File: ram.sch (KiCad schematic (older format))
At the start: 7 parts, among them U1 LFE5U-85F-6BG381C

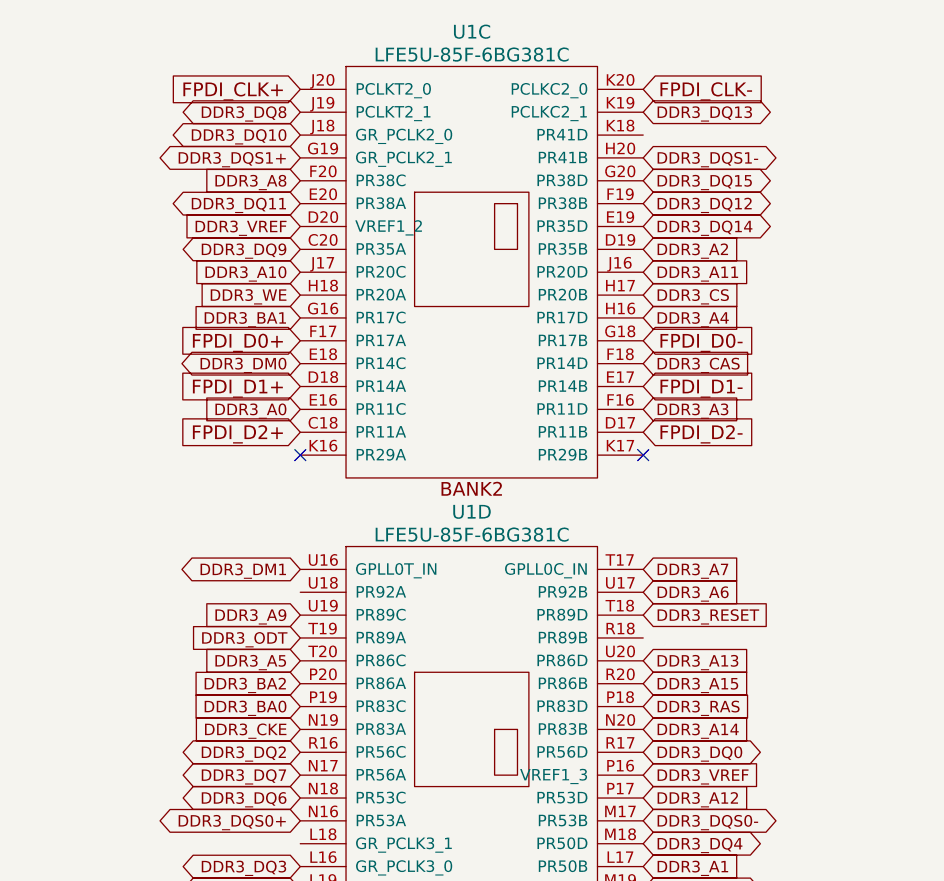
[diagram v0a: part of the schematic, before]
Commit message: Diff pair length done
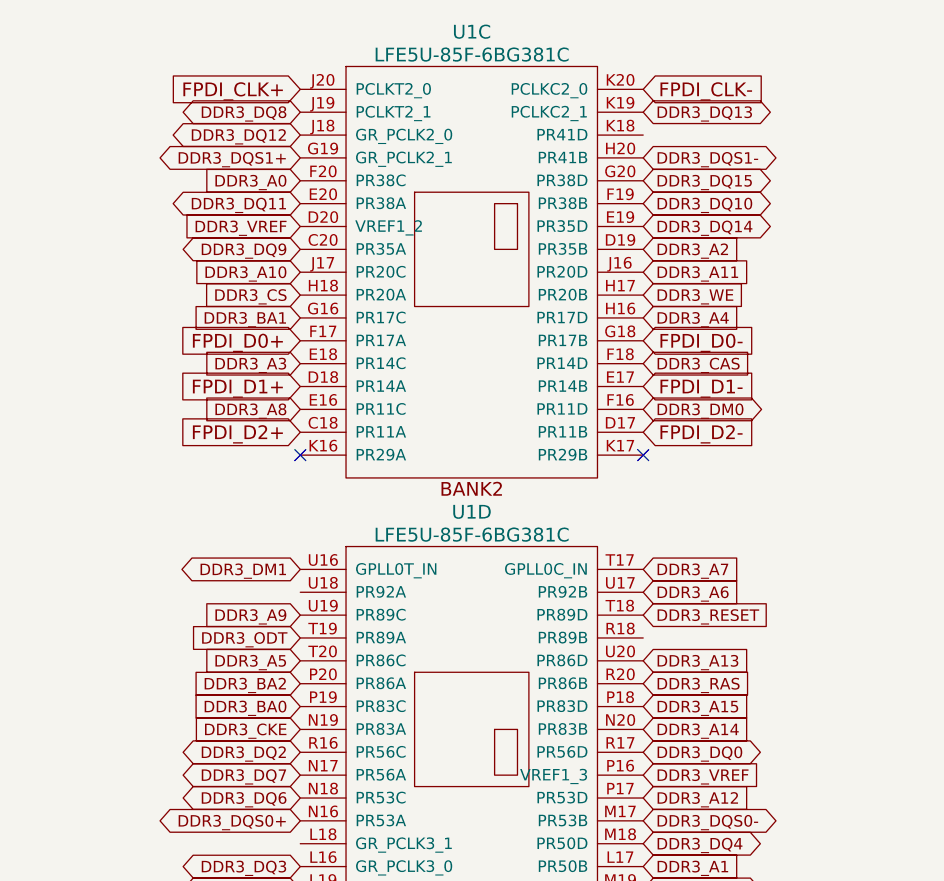
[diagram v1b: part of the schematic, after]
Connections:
- net DDR3_A0: now also U1.F20 (PR38C); no longer U1.E16 (PR11C)
- net DDR3_A15: now also U1.P18 (PR83D); no longer U1.R20 (PR86B)
- net DDR3_A3: now also U1.E18 (PR14C); no longer U1.F16 (PR11D)
- net DDR3_A8: now also U1.E16 (PR11C); no longer U1.F20 (PR38C)
- net DDR3_CS: now also U1.H18 (PR20A); no longer U1.H17 (PR20B)
- net DDR3_DM0: now also U1.F16 (PR11D); no longer U1.E18 (PR14C)
- net DDR3_DQ10: now also U1.F19 (PR38B); no longer U1.J18 (GR_PCLK2_0)
- net DDR3_DQ12: now also U1.J18 (GR_PCLK2_0); no longer U1.F19 (PR38B)
- net DDR3_RAS: now also U1.R20 (PR86B); no longer U1.P18 (PR83D)
- net DDR3_WE: now also U1.H17 (PR20B); no longer U1.H18 (PR20A)
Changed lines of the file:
@@
 Text GLabel 8100 2400 2    50   Input ~ 0
 DDR3_A2
-Text GLabel 8100 3100 2    50   Input ~ 0
+Text GLabel 6600 2900 0    50   Input ~ 0
 DDR3_A3
 Text GLabel 8100 2700 2    50   Input ~ 0
@@
 Text GLabel 8100 3800 2    50   Input ~ 0
 DDR3_A7
-Text GLabel 6600 2100 0    50   Input ~ 0
+Text GLabel 6600 3100 0    50   Input ~ 0
 DDR3_A8
 Text GLabel 6600 4000 0    50   Input ~ 0
@@
 Text GLabel 8100 4000 2    50   Input ~ 0
 DDR3_RESET
-Text GLabel 8100 2600 2    50   Input ~ 0
+Text GLabel 6600 2600 0    50   Input ~ 0
 DDR3_CS
 Text GLabel 8100 2900 2    50   Input ~ 0
 DDR3_CAS
-Text GLabel 8100 4400 2    50   Input ~ 0
+Text GLabel 8100 4300 2    50   Input ~ 0
 DDR3_RAS
-Text GLabel 6600 2600 0    50   Input ~ 0
+Text GLabel 8100 2600 2    50   Input ~ 0
 DDR3_WE
 Text GLabel 6600 4100 0    50   Input ~ 0
@@
 Text GLabel 6600 4700 0    50   BiDi ~ 0
 DDR3_DQ7
-Text GLabel 6600 1900 0    50   BiDi ~ 0
+Text GLabel 8100 2200 2    50   BiDi ~ 0
 DDR3_DQ10
 Text GLabel 6600 2200 0    50   BiDi ~ 0
 DDR3_DQ11
-Text GLabel 8100 2200 2    50   BiDi ~ 0
+Text GLabel 6600 1900 0    50   BiDi ~ 0
 DDR3_DQ12
 Text GLabel 8100 2300 2    50   BiDi ~ 0
@@
 Text GLabel 8100 4900 2    50   BiDi ~ 0
 DDR3_DQS0-
-Text GLabel 8100 4300 2    50   Input ~ 0
+Text GLabel 8100 4400 2    50   Input ~ 0
 DDR3_A15
 Text GLabel 6600 4200 0    50   Input ~ 0
@@
 Text GLabel 8100 1800 2    50   BiDi ~ 0
 DDR3_DQ13
-Text GLabel 6600 2900 0    50   BiDi ~ 0
+Text GLabel 8100 3100 2    50   BiDi ~ 0
 DDR3_DM0
 Text GLabel 6600 2300 0    50   Input ~ 0
@@
 Text GLabel 6600 1800 0    50   BiDi ~ 0
 DDR3_DQ8
-Text GLabel 6600 3100 0    50   Input ~ 0
+Text GLabel 6600 2100 0    50   Input ~ 0
 DDR3_A0
 Text GLabel 6600 2000 0    50   BiDi ~ 0

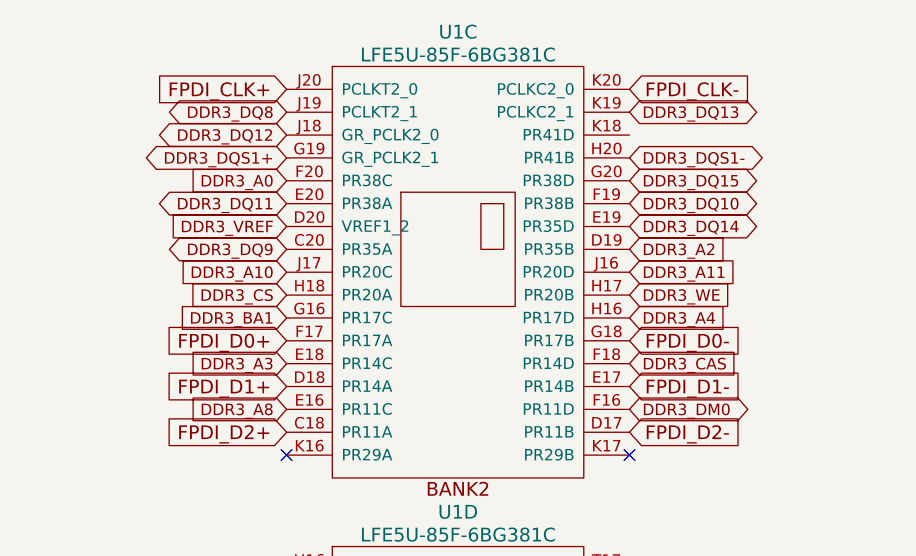
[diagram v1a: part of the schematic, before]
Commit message: Almost to 10%
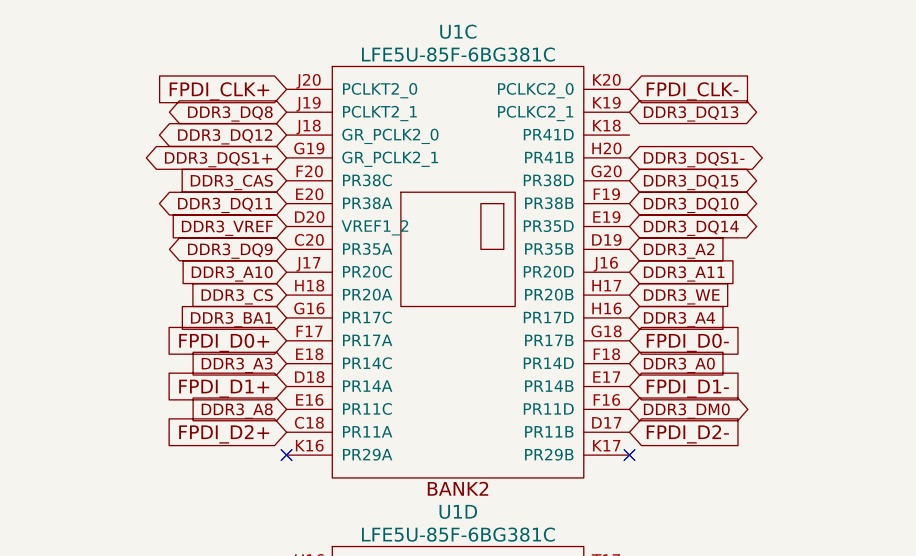
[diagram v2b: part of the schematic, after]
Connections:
- net DDR3_A0: now also U1.F18 (PR14D); no longer U1.F20 (PR38C)
- net DDR3_CAS: now also U1.F20 (PR38C); no longer U1.F18 (PR14D)
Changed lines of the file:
@@
 Text GLabel 6600 2600 0    50   Input ~ 0
 DDR3_CS
-Text GLabel 8100 2900 2    50   Input ~ 0
+Text GLabel 6600 2100 0    50   Input ~ 0
 DDR3_CAS
 Text GLabel 8100 4300 2    50   Input ~ 0
@@
 Text GLabel 6600 1800 0    50   BiDi ~ 0
 DDR3_DQ8
-Text GLabel 6600 2100 0    50   Input ~ 0
+Text GLabel 8100 2900 2    50   Input ~ 0
 DDR3_A0
 Text GLabel 6600 2000 0    50   BiDi ~ 0
